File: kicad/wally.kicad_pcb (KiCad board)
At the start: 4 copper layers, 50 x 30 mm, 36 parts, among them J1 USB C, J2 HDMI_A, J3 HDMI_A, J4 Debug, Q1 AO3401A, Q2 AO3401A, Q3 AO3401A, Q4 AO3400A, SW1 Boot, U1 STM32F042F6Px, U2 XC6206PxxxMR, U3 SRV05-4

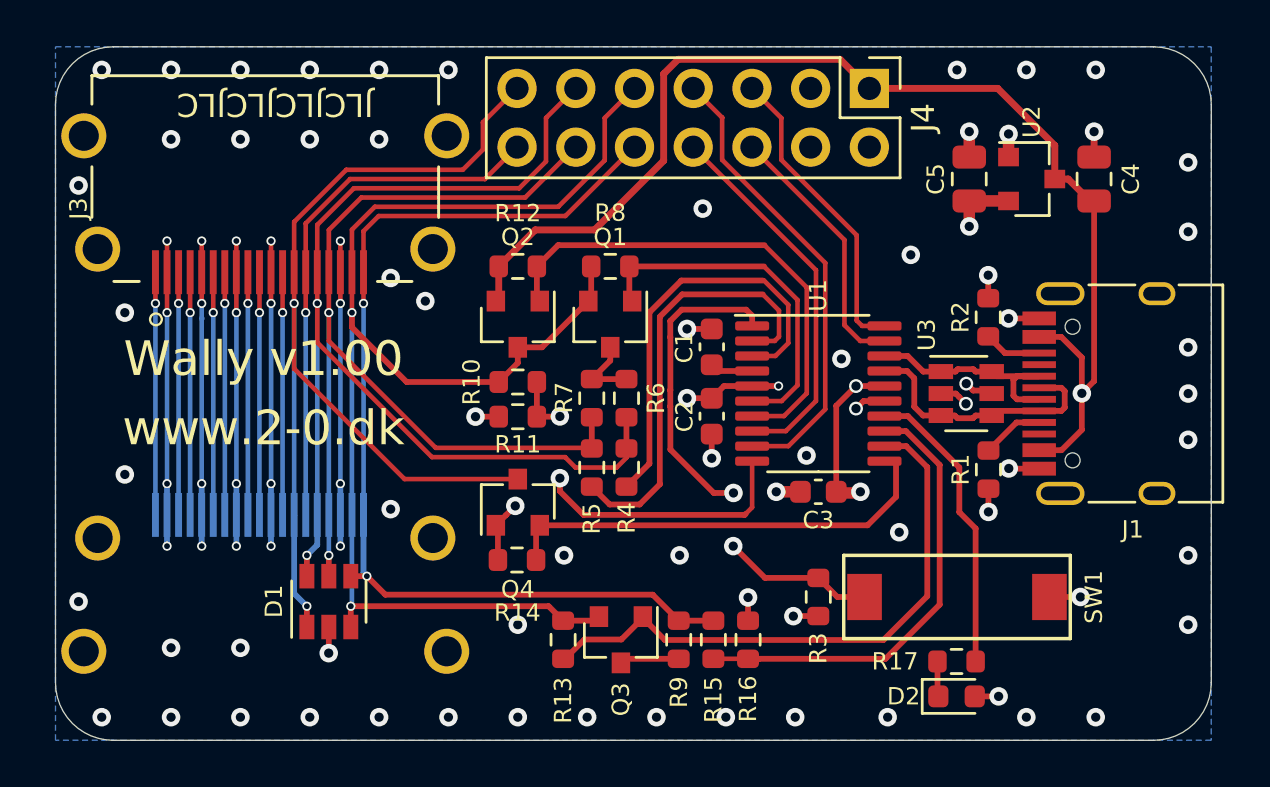
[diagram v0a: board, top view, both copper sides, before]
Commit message: Wally v1.01
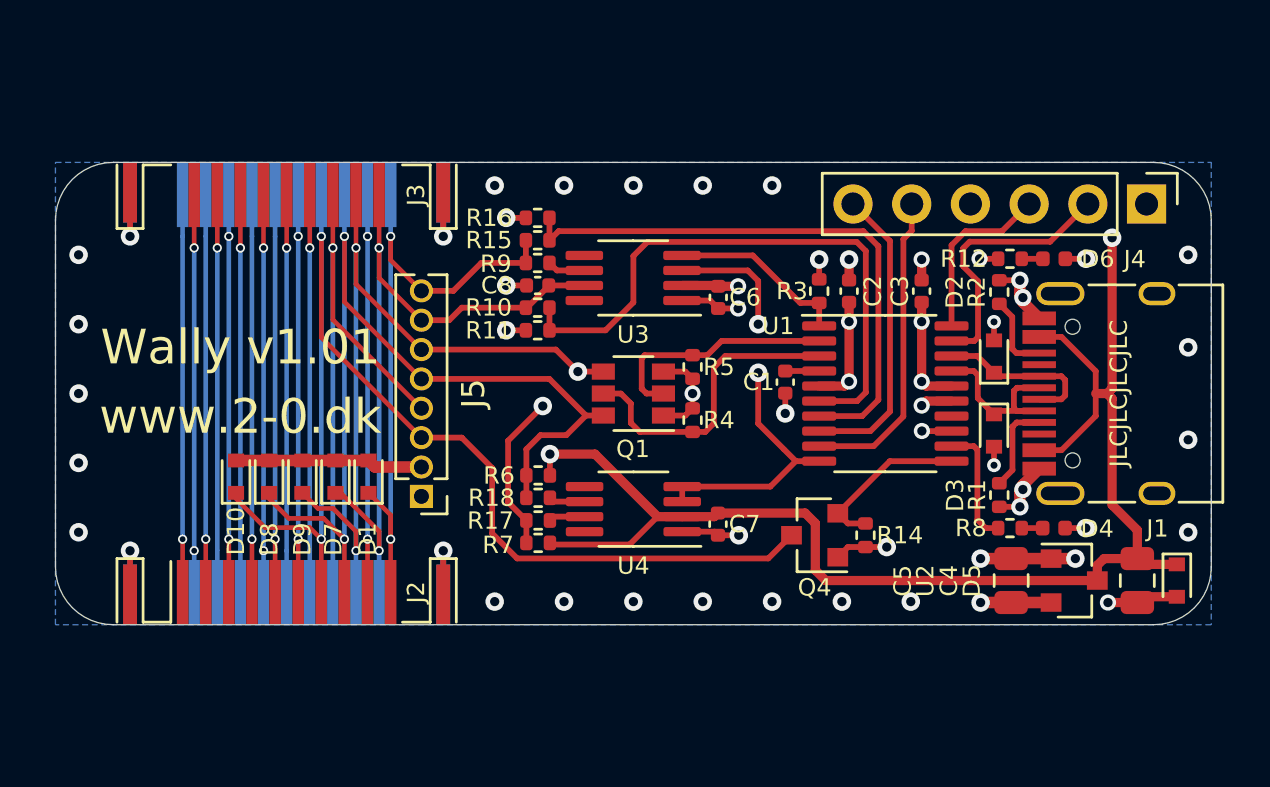
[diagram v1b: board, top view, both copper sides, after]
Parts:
- removed Q2, Q3: AO3401A, Package_TO_SOT_SMD:SOT-23
- removed R13: 10k, Resistor_SMD:R_0603_1608Metric
- removed SW1: Boot, wally:TACT-SWITCH
- added C6: 100n, Capacitor_SMD:C_0402_1005Metric, F.Cu at (153.7, 95.8)
- added C7: 100n, Capacitor_SMD:C_0402_1005Metric, F.Cu at (153.7, 105.7)
- added C8: 100n, Capacitor_SMD:C_0402_1005Metric, F.Cu at (145.9, 95.3)
- added D10: ESD5Z5.0, Diode_SMD:D_SOD-523, F.Cu at (132.8, 103.6)
- added D3: ESD5Z5.0, Diode_SMD:D_SOD-523, F.Cu at (165.6, 101.6)
- added D4: LED, LED_SMD:LED_0402_1005Metric, F.Cu at (168.2, 105.8)
- added D5: ESD5Z5.0, Diode_SMD:D_SOD-523, F.Cu at (173.5, 108.1)
- added D6: LED, LED_SMD:LED_0402_1005Metric, F.Cu at (168.2, 94.2)
- added D7: ESD5Z5.0, Diode_SMD:D_SOD-523, F.Cu at (137.1, 103.6)
- added D8: ESD5Z5.0, Diode_SMD:D_SOD-523, F.Cu at (134.2, 103.6)
- added D9: ESD5Z5.0, Diode_SMD:D_SOD-523, F.Cu at (135.7, 103.6)
- added J5: HDMI Expansion, Connector_PinHeader_1.27mm:PinHeader_1x08_P1.27mm_Vertical, F.Cu at (140.8, 104.4)
- added R18: 1k5, Resistor_SMD:R_0402_1005Metric, F.Cu at (145.9, 104.5)
- added U4: AP2152, Package_SO:MSOP-8_3x3mm_P0.65mm, F.Cu at (150.0, 105.0)
- C1, C2, C3: footprint Capacitor_SMD:C_0603_1608Metric -> Capacitor_SMD:C_0402_1005Metric
- C5: value 1u -> 10u
- D1: value SP0505BAHT -> ESD5Z5.0; footprint Package_TO_SOT_SMD:SOT-23-6 -> Diode_SMD:D_SOD-523
- D2: value LED -> ESD5Z5.0; footprint LED_SMD:LED_0603_1608Metric -> Diode_SMD:D_SOD-523
- J2: footprint wally:AMPHENOL_10029449-001RLF -> Connector_HDMI:HDMI_A_Contact_Technology_HDMI-19APL2_Horizontal; moved to F.Cu
- J3: footprint wally:AMPHENOL_10029449-001RLF -> Connector_HDMI:HDMI_A_Contact_Technology_HDMI-19APL2_Horizontal; moved to B.Cu
- J4: footprint Connector_PinHeader_2.54mm:PinHeader_2x07_P2.54mm_Vertical -> Connector_PinHeader_2.54mm:PinHeader_1x06_P2.54mm_Vertical
- Q1: value AO3401A -> NDC7002N; footprint Package_TO_SOT_SMD:SOT-23 -> Package_TO_SOT_SMD:SuperSOT-6
- R1, R14, R2, R3, R9: footprint Resistor_SMD:R_0603_1608Metric -> Resistor_SMD:R_0402_1005Metric
- R10, R15: value 20k -> 40k; footprint Resistor_SMD:R_0603_1608Metric -> Resistor_SMD:R_0402_1005Metric
- R11, R16: value 30k -> 60k; footprint Resistor_SMD:R_0603_1608Metric -> Resistor_SMD:R_0402_1005Metric
- R12, R8: value 10k -> 1k; footprint Resistor_SMD:R_0603_1608Metric -> Resistor_SMD:R_0402_1005Metric
- R17: value 1k -> 1k5; footprint Resistor_SMD:R_0603_1608Metric -> Resistor_SMD:R_0402_1005Metric
- R4, R5: value 100 -> 20k; footprint Resistor_SMD:R_0603_1608Metric -> Resistor_SMD:R_0402_1005Metric
- R6, R7: value 1k5 -> 100k; footprint Resistor_SMD:R_0603_1608Metric -> Resistor_SMD:R_0402_1005Metric
- U3: value SRV05-4 -> AP2152; footprint Package_TO_SOT_SMD:SOT-23-6 -> Package_SO:MSOP-8_3x3mm_P0.65mm
- moved R12 21.3 mm to (166.3, 94.2)
- moved R8 20.7 mm to (166.3, 105.8)
- moved R16 20.4 mm to (145.9, 92.4), turned to 180 degrees
- moved R17 19.1 mm to (145.9, 105.5)
- moved R15 18.9 mm to (145.9, 93.4), turned to 0 degrees
- moved C4 17.5 mm to (171.8, 108.1), turned to 90 degrees
- moved U2 17.5 mm to (169.1, 108.1)
- moved C5 17.5 mm to (166.3, 108.1)
- moved R9 17.4 mm to (145.9, 94.3), turned to 180 degrees
- moved U3 15.3 mm to (150.0, 95.0), turned to 180 degrees
- moved R14 15.1 mm to (160.0, 106.1), turned to 90 degrees
- moved D2 14.8 mm to (165.6, 98.4), turned to 90 degrees
- moved R3 13.2 mm to (158.0, 95.6), turned to 90 degrees
- moved J4 13.0 mm to (172.2, 91.8)
- moved Q4 12.9 mm to (157.8, 106.1), turned to 180 degrees
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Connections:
- D1 pad 1: hdmi_cec -> hdmi_hpd
- D2 pad 1: Net-(D2-Pad1) -> usb_dp
- D2 pad 2: +3V3 -> GND
- J1 pad S1: Net-(J1-PadS1) -> (no net)
- J4 pad 1: +5V -> GND
- J4 pad 2: +3V3 -> swdio
- J4 pad 3: GND -> swclk
- J4 pad 5: swclk -> uart_rx
- J4 pad 6: swdio -> uart_tx
- Q1 pad 1: hdmi_i2c_en -> +3V3
- Q1 pad 2: hdmi_5v -> i2c_sda
- Q1 pad 3: Net-(Q1-Pad3) -> +3V3
- R12 pad 1: +5V -> Net-(R12-Pad1)
- R12 pad 2: hdmi_5v_en -> Net-(D6-Pad2)
- R17 pad 1: led0 -> Net-(R17-Pad1)
- R17 pad 2: Net-(D2-Pad1) -> hdmi_sda
- R3 pad 1: boot -> hdmi_hpd_en
- R4 pad 1: hdmi_scl -> +3V3
- R5 pad 1: hdmi_sda -> +3V3
- R6 pad 1: Net-(Q1-Pad3) -> +5V
- R7 pad 1: Net-(Q1-Pad3) -> +5V
- R8 pad 1: hdmi_5v -> Net-(R8-Pad1)
- R8 pad 2: hdmi_i2c_en -> Net-(D4-Pad2)
- R9 pad 1: Net-(Q3-Pad3) -> Net-(R9-Pad1)
- U1 pad 1: boot -> hdmi_hpd_en
- U1 pad 10: hdmi_5v_in -> hdmi_5v_en
- U1 pad 12: hdmi_hpd_en -> Net-(R8-Pad1)
- U1 pad 13: hdmi_hpd_in -> Net-(R12-Pad1)
- U1 pad 14: led0 -> (no net)
- U1 pad 6: hdmi_i2c_en -> hdmi_5v_in
- U1 pad 7: hdmi_5v_en -> hdmi_hpd_in
- U3 pad 1: usb_dp -> GND
- U3 pad 2: GND -> +5V
- U3 pad 3: usb_dm -> hdmi_5v_en
- U3 pad 4: usb_dm -> hdmi_hpd_en
- U3 pad 5: +5V -> (no net)
- U3 pad 6: usb_dp -> Net-(R9-Pad1)
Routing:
- net GND: track 98.2 -> 165.8 mm, vias 87 -> 56
- net +5V: track 59.3 -> 86.8 mm, vias 2 -> 3
- net hdmi_5v: track 59.3 -> 32.2 mm
- net boot: track 22.3 -> 0.00 mm, vias 2 -> 0
- net hdmi_hpd_en: track 25.0 -> 7.78 mm
- net Net-(J1-PadS1): track 17.0 -> 0.00 mm
- net hdmi_hpd: track 44.7 -> 28.5 mm
- net hdmi_i2c_en: track 15.4 -> 0.00 mm
- net led0: track 12.3 -> 0.00 mm
- net hdmi_cec_in: track 19.0 -> 7.24 mm
- net Net-(R12-Pad1): track 0.00 -> 11.5 mm, vias 0 -> 2
- net hdmi_5v_in: track 16.6 -> 25.9 mm, vias 2 -> 0
- net i2c_sda: track 19.1 -> 10.3 mm
- net hdmi_cec: track 45.0 -> 52.4 mm
- net hdmi_scl: track 49.3 -> 42.5 mm
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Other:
- board size 50 x 30 mm -> 50 x 20 mm
- board text added: "GND"
- board text added: "RX"
- board text added: "SWCLK"
- board text added: "SWDIO"
- board text added: "TX"
- board text added: "Wally v1.01"
- board text removed: "Wally v1.00"
